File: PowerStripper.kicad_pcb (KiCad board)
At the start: 2 copper layers, 37.3 x 31 mm, 5 parts, among them J1 0548190519, J2 UE27AC54100

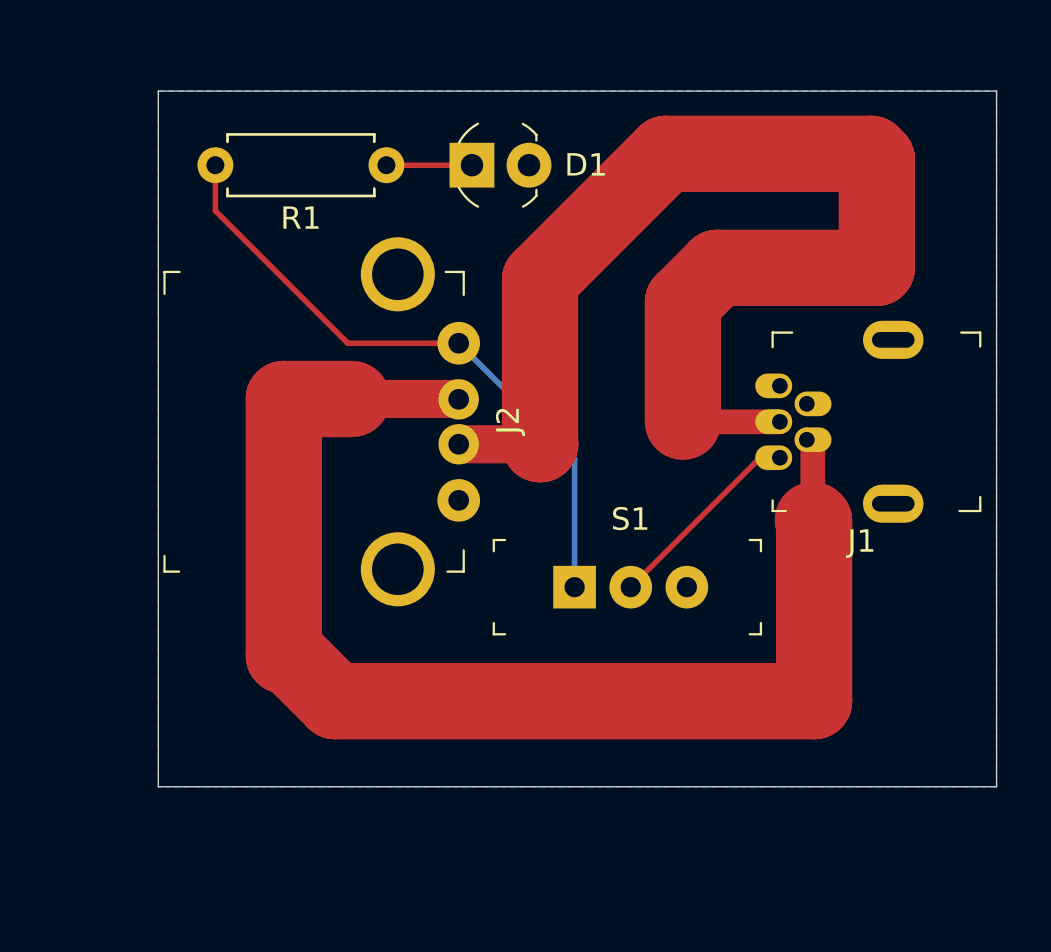
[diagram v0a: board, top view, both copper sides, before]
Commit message: So close, yet so far
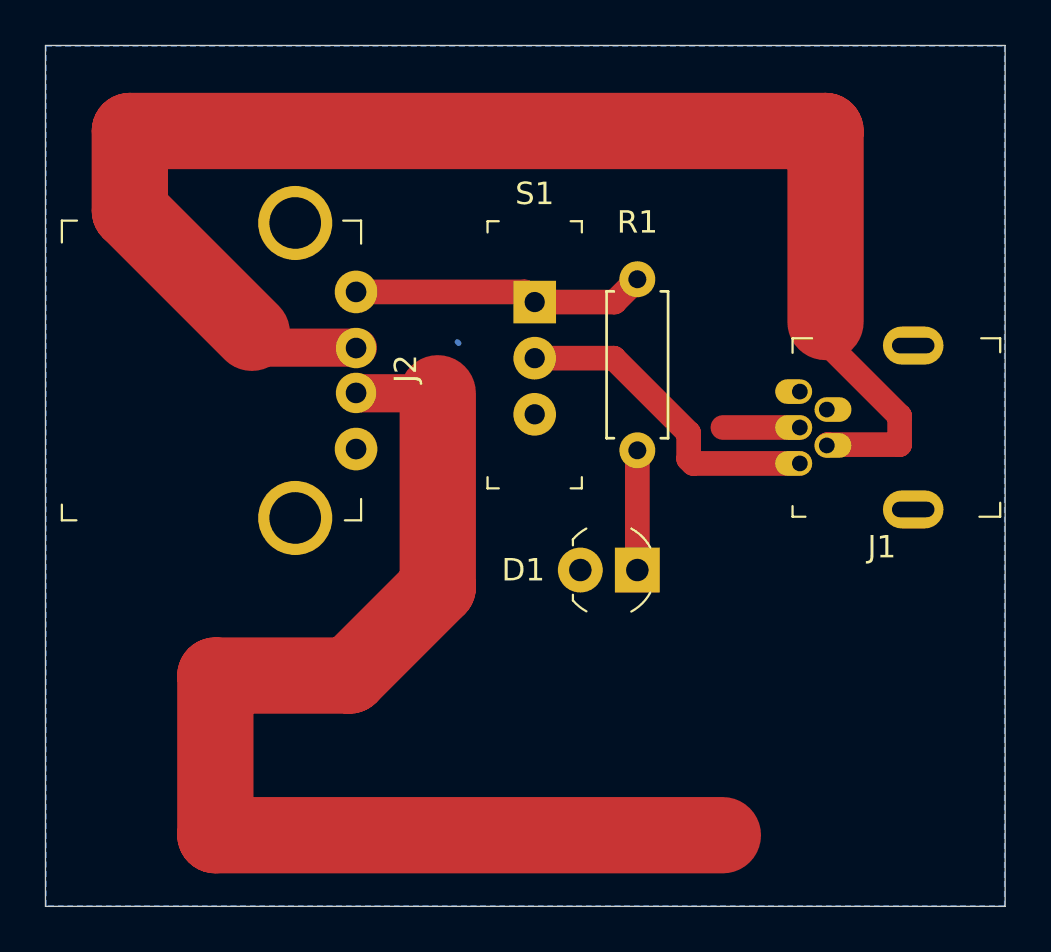
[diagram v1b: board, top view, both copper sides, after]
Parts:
- moved D1 18.2 mm to (116.3, 112.3), turned to 180 degrees
- moved R1 16.9 mm to (118.9, 106.9), turned to 90 degrees
- moved S1 12.8 mm to (114.3, 100.3), turned to 270 degrees
- moved J2 5.11 mm to (103.6, 103.4)
- moved J1 0.92 mm to (126.1, 105.9)
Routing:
- net Net-(J2-Pad1): track 28.5 -> 13.1 mm
- net D-: track 55.5 -> 65.6 mm
- net Net-(J1-Pad1): track 9.91 -> 15.3 mm
- net D+: track 52.2 -> 57.1 mm
- net Net-(D1-Pad1): track 3.81 -> 5.33 mm
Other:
- board size 37.3 x 31 mm -> 42.7 x 38.3 mm
- rule trace_min: 0.152 -> 0.1524
